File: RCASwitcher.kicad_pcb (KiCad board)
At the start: 2 copper layers, 144.5 x 76 mm, 17 parts, among them J1 Connector_RCA_2x3_REB, J2 Connector_RCA_2x3_REB, J3 Connector_RCA_2x3_REB, J4 Connector_RCA_2x3_REB, J5 Connector_RCA_2x3_REB, J6 Connector_RCA_2x3_REB, SW1 SW_SPDT_3x2_REB, SW2 SW_SPDT_3x2_REB, SW3 SW_SPDT_3x2_REB, SW4 SW_SPDT_3x2_REB, SW5 SW_SPDT_3x2_REB

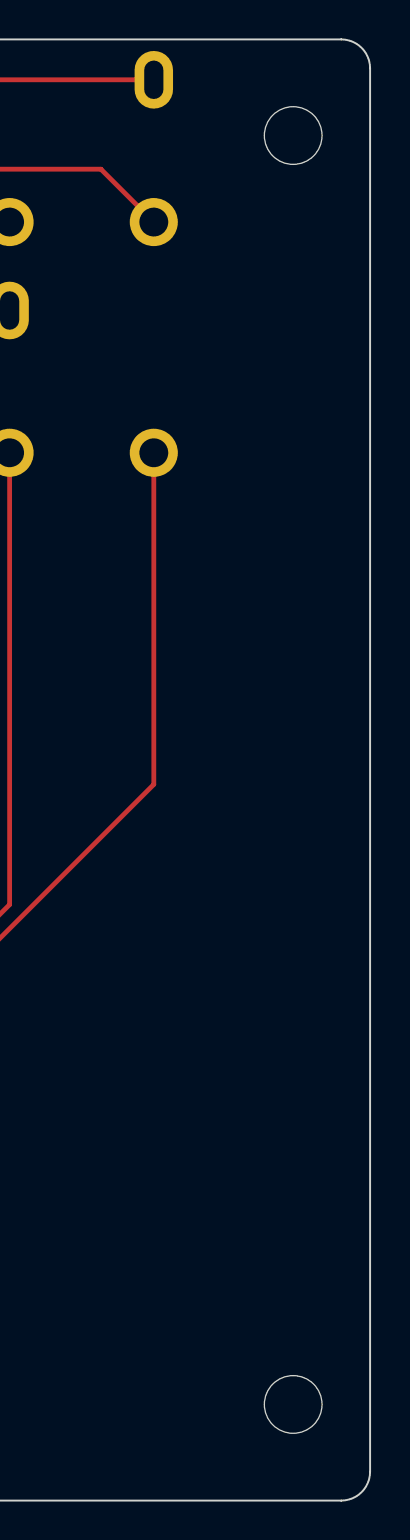
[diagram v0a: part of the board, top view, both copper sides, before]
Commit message: Adds 3d model and gerbers for fabrication
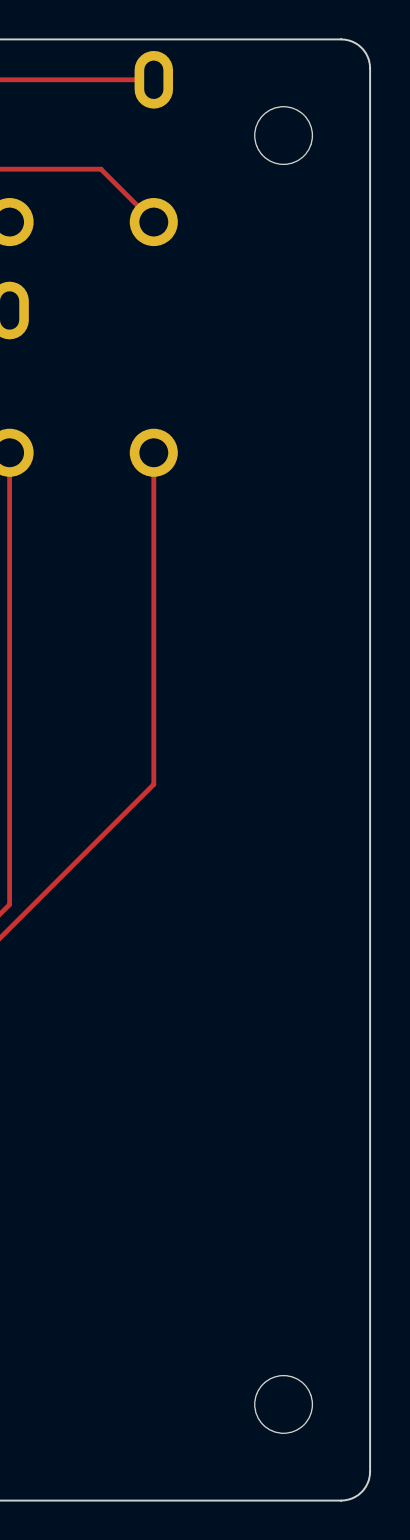
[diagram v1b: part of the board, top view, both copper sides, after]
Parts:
- moved REF** 0.50 mm to (163.5, 136.0)
- moved REF** 0.50 mm to (163.5, 70.0)
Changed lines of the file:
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@@
   )
   (footprint "MountingHole:MountingHole_3mm" (layer "F.Cu")
-    (at 164 136)
+    (at 163.5 136)
     (descr "Mounting Hole 3mm, no annular")
     (tags "mounting hole 3mm no annular")
@@
   )
   (footprint "MountingHole:MountingHole_3mm" (layer "F.Cu")
-    (at 164 70)
+    (at 163.5 70)
     (descr "Mounting Hole 3mm, no annular")
     (tags "mounting hole 3mm no annular")
